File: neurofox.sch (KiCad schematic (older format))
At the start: 1 part

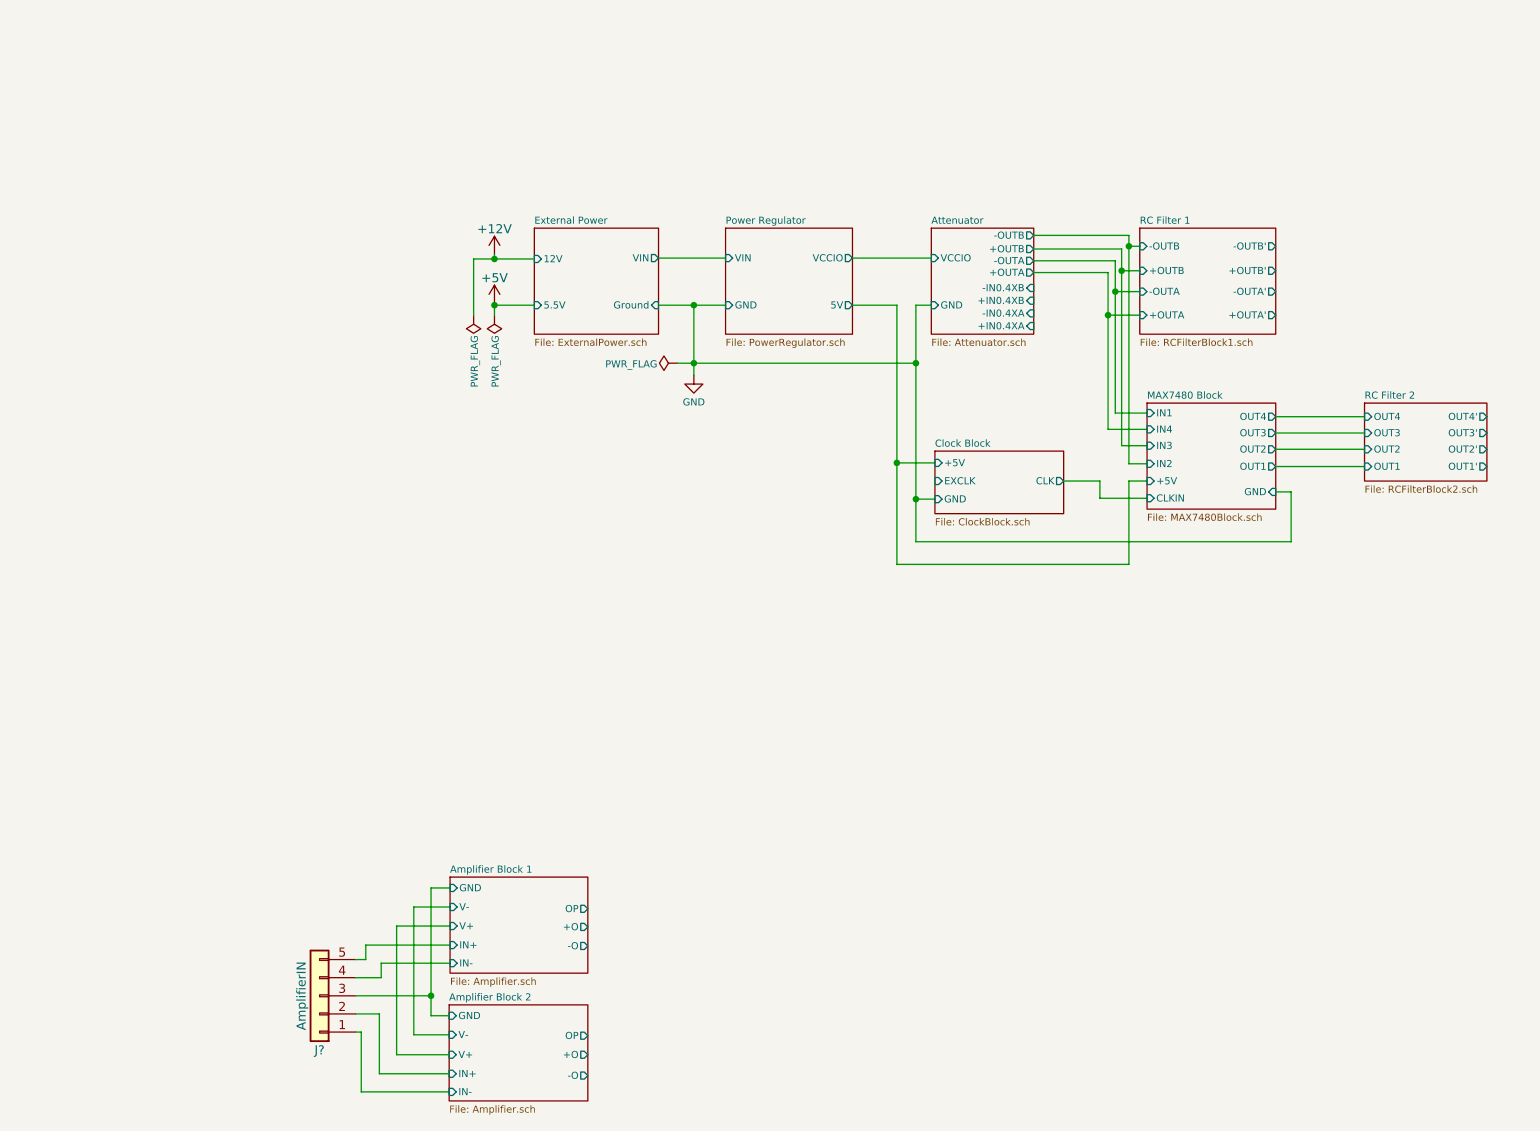
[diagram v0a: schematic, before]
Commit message: feat: alignment
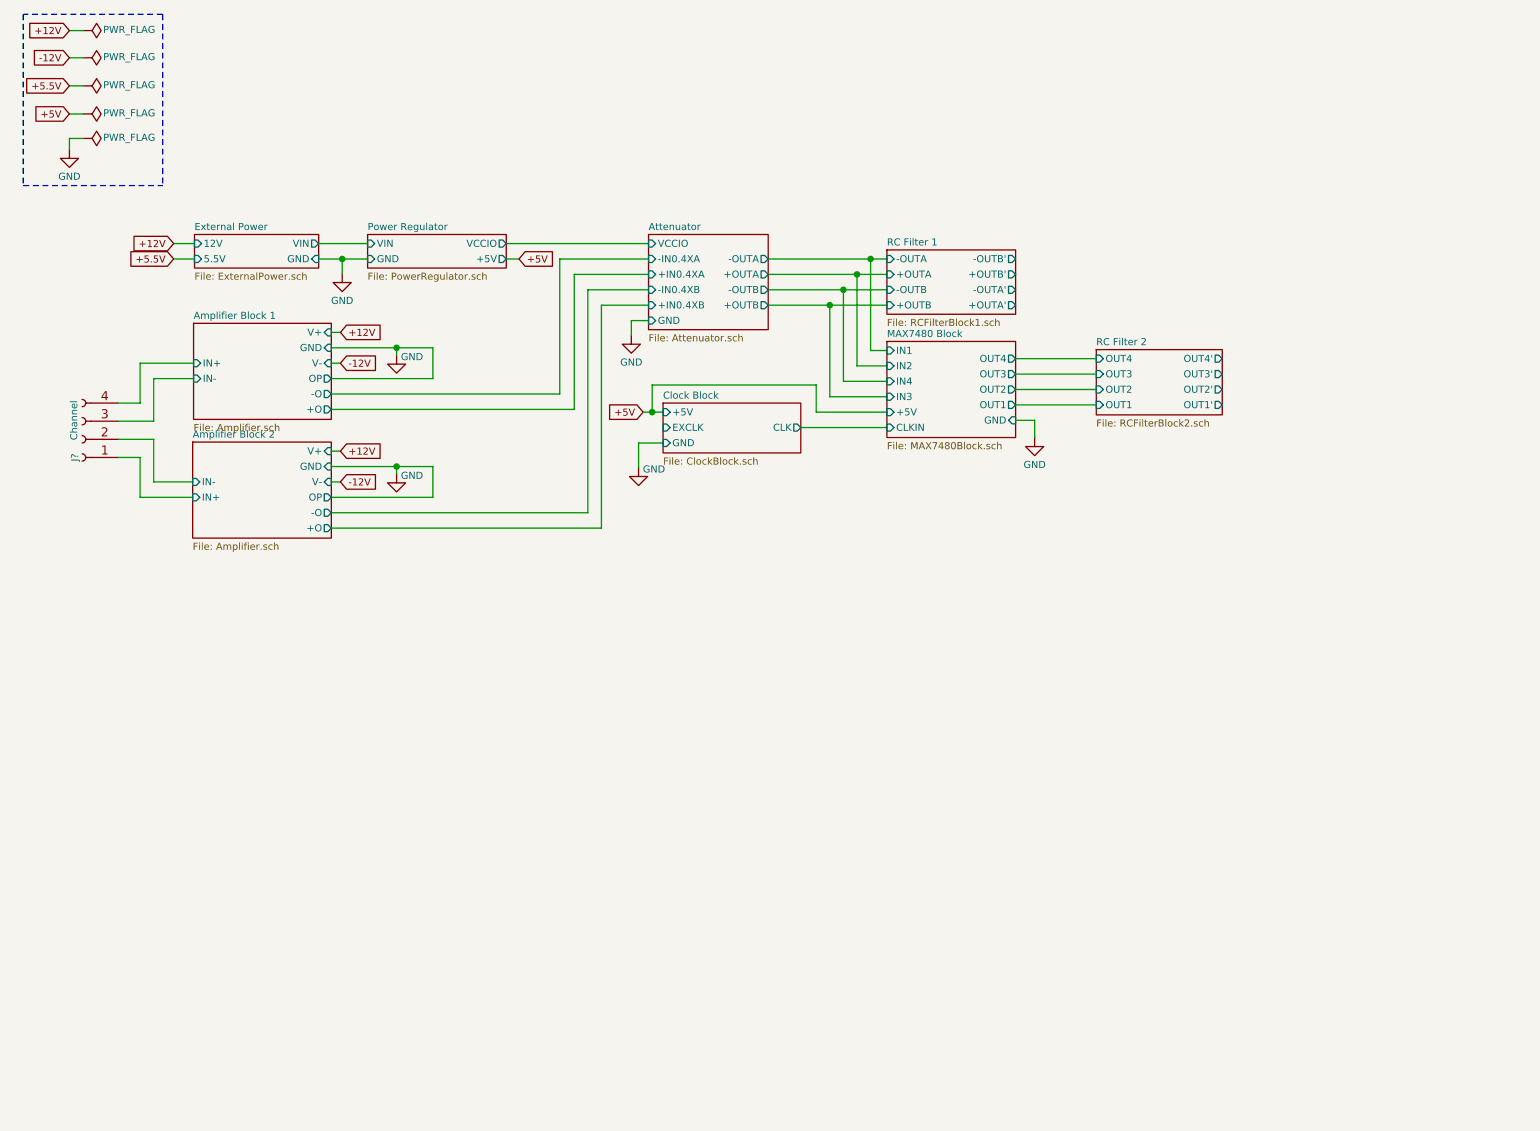
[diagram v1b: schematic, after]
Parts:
- removed J?: AmplifierIN, symbol Conn_01x05
- added J?: Channel, symbol Conn_01x04_Female
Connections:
- net Amplifier Block 1/IN+: now also J?.4 (Pin_4)
- net Amplifier Block 1/IN-: now also J?.3 (Pin_3)
- net Amplifier Block 2/IN+: now also J?.1 (Pin_1)
- net Amplifier Block 2/IN-: now also J?.2 (Pin_2)
